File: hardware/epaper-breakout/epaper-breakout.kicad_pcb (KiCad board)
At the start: 2 copper layers, 100 x 40.5 mm, 90 parts, among them J1 XF2M-3315-1A, J2 C10418, J3 Conn_02x06_Counter_Clockwise, J4 ED060SC4, J5 Conn_01x01_Male, J6 Conn_01x01_Male, Q1 AO3401A, Q2 AO3401A, Q3 MMBT3904, Q4 MMBT3904, Q5 AO3401A, Q6 MMBT3904, U1 MCP1700-3302E_SOT23, U10 ED060SC7, U11 TP4056, U12 CH340C, U2 LT1945, U3 LT1945, U4 XC6206PxxxMR, U5 ESP32-WROVER, U6 ED060XC5, U7 LM358, U8 74HC4094-normal, U9 MCP9700AT-ETT

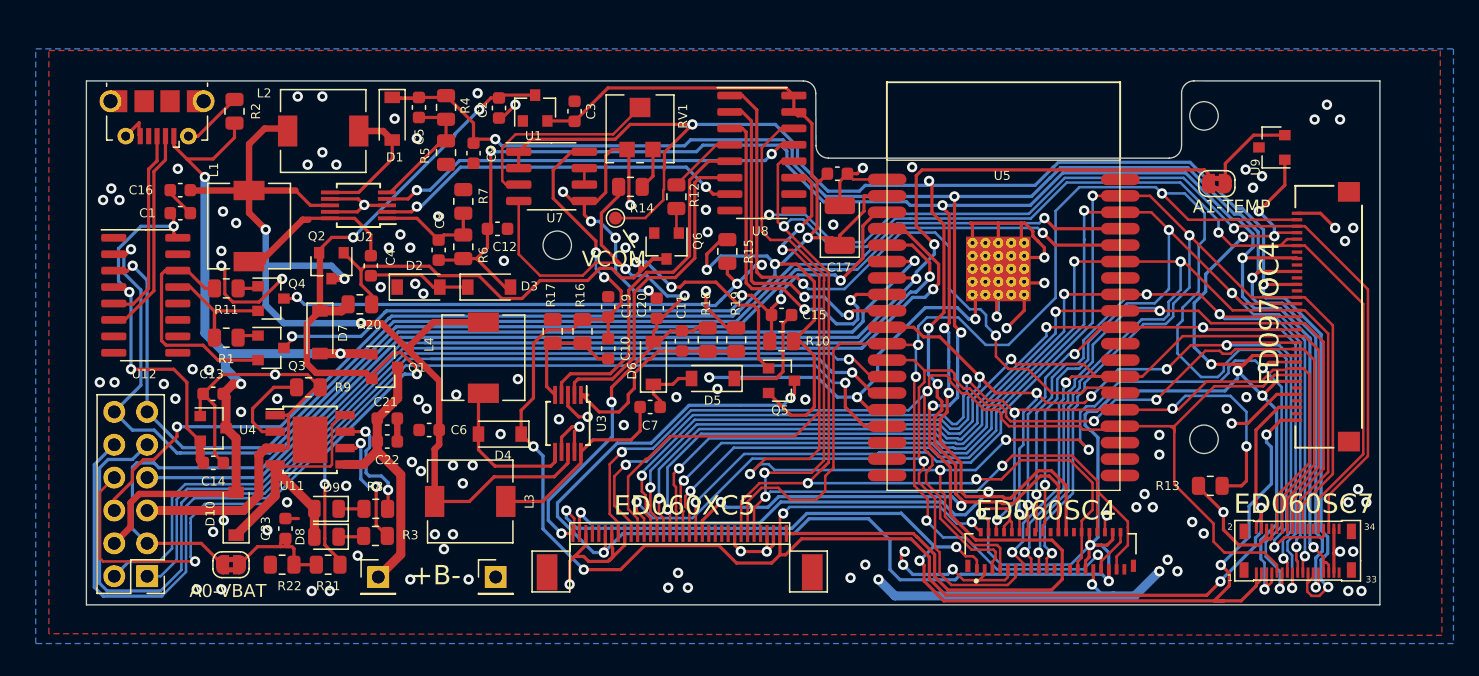
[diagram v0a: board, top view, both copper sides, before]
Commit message: pcb routing
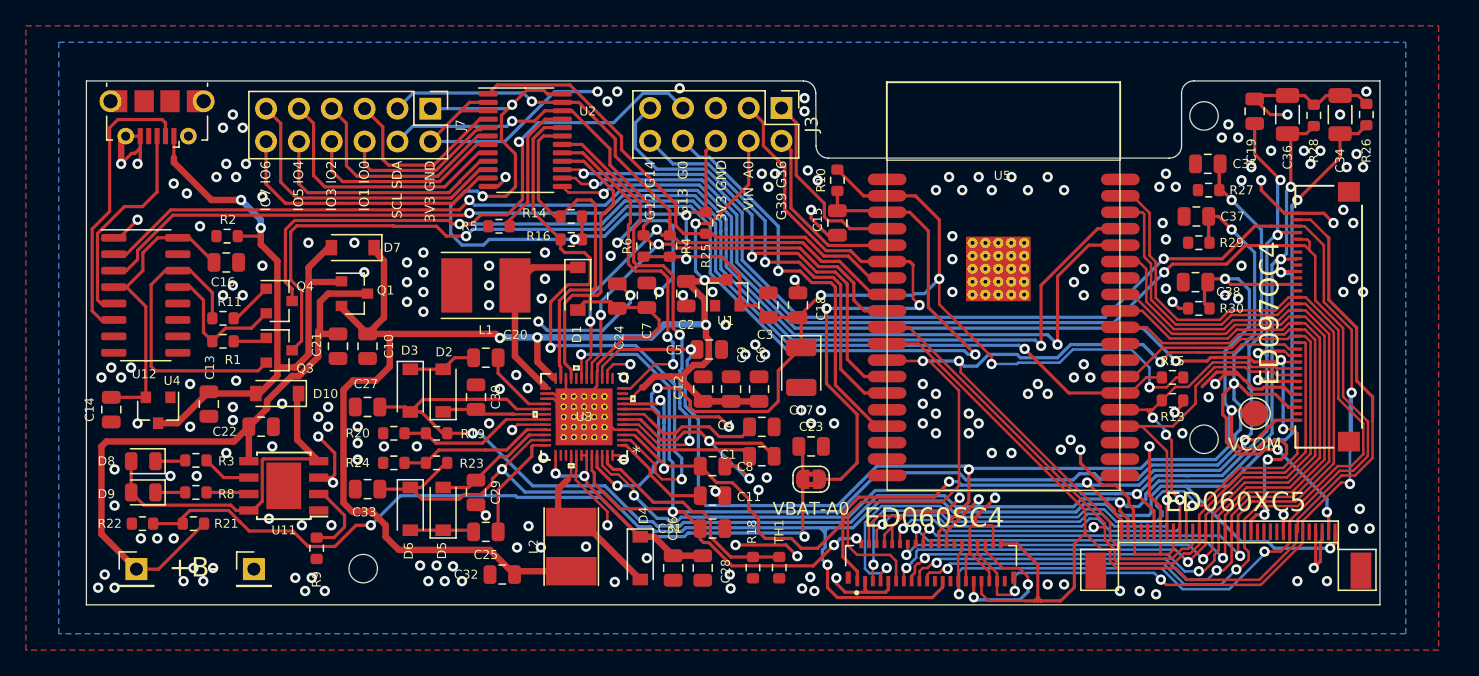
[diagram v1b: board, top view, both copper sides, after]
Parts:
- removed JP_TEMP1: Jumper, Jumper:SolderJumper-2_P1.3mm_Bridged2Bar_RoundedPad1.0x1.5mm
- removed L3, L4: 22uH, Inductor_SMD:L_6.3x6.3_H3
- removed Q2, Q5: AO3401A, Package_TO_SOT_SMD:SOT-23
- removed Q6: MMBT3904, Package_TO_SOT_SMD:SOT-23
- removed R12: 1k, Resistor_SMD:R_0805_2012Metric
- removed R17: 27k, Resistor_SMD:R_0805_2012Metric
- removed R7: 39k, Resistor_SMD:R_0805_2012Metric
- removed RV1: 200k, epaper-breakout:EVM3ESX50B25
- removed TP1: TestPoint_Probe, TestPoint:TestPoint_Pad_D1.0mm
- removed U10: ED060SC7, epaper-breakout:AXT334124
- removed U7: LM358, Package_SO:SOP-8_3.76x4.96mm_P1.27mm
- removed U8: 74HC4094-normal, Package_SO:SOIC-16_3.9x9.9mm_P1.27mm
- removed U9: MCP9700AT-ETT, Package_TO_SOT_SMD:SOT-23
- added C24: 4.7uF, Capacitor_SMD:C_0805_2012Metric, F.Cu at (66.0, 36.1)
- added C25: 10nF, Capacitor_SMD:C_0805_2012Metric, F.Cu at (55.9, 54.4)
- added C26: 4.7uF, Capacitor_SMD:C_0805_2012Metric, F.Cu at (70.4, 57.1)
- added C27: 2.2uF, Capacitor_SMD:C_0805_2012Metric, F.Cu at (46.7, 44.7)
- added C28: 4.7uF, Capacitor_SMD:C_0805_2012Metric, F.Cu at (72.6, 57.1)
- added C29: 100nF, Capacitor_SMD:C_0805_2012Metric, F.Cu at (55.1, 51.3)
- added C30: 100nF, Capacitor_SMD:C_0805_2012Metric, F.Cu at (55.1, 43.9)
- added C31: 4.7uF, Capacitor_SMD:C_0805_2012Metric, F.Cu at (73.4, 54.1)
- added C32: 10uF, Capacitor_SMD:C_0805_2012Metric, F.Cu at (57.1, 57.7)
- added C33: 2.2uF, Capacitor_SMD:C_0805_2012Metric, F.Cu at (46.7, 51.1)
- added C34: 1uF/50V, Capacitor_SMD:C_1206_3216Metric, F.Cu at (121.9, 22.1)
- added C35: 1uF/25V, Capacitor_SMD:C_0805_2012Metric, F.Cu at (111.7, 25.9)
- added C36: 1uF/50V, Capacitor_SMD:C_1206_3216Metric, F.Cu at (117.9, 22.1)
- added C37: 1uF/25V, Capacitor_SMD:C_0805_2012Metric, F.Cu at (110.8, 30.0)
- added C38: 1uF/25V, Capacitor_SMD:C_0805_2012Metric, F.Cu at (110.7, 35.1)
- added J7: Conn_01x12, Connector_PinHeader_2.54mm:PinHeader_2x06_P2.54mm_Vertical, F.Cu at (51.6, 21.6)
- added R23: 1M, Resistor_SMD:R_0603_1608Metric, F.Cu at (52.1, 49.0)
- added R24: 47.5k, Resistor_SMD:R_0603_1608Metric, F.Cu at (48.8, 49.0)
- added R25: 10k, Resistor_SMD:R_0603_1608Metric, F.Cu at (72.9, 30.5)
- added R26: 47k, Resistor_SMD:R_0603_1608Metric, F.Cu at (124.0, 22.1)
- added R27: 47k, Resistor_SMD:R_0603_1608Metric, F.Cu at (111.8, 27.9)
- added R28: 47k, Resistor_SMD:R_0603_1608Metric, F.Cu at (119.9, 22.2)
- added R29: 47k, Resistor_SMD:R_0603_1608Metric, F.Cu at (111.0, 32.0)
- added R30: 100k, Resistor_SMD:R_0603_1608Metric, F.Cu at (111.0, 37.1)
- added TH1: 10k, Resistor_SMD:R_0603_1608Metric, F.Cu at (78.6, 57.1)
- added TP_VCOM1: VCOM, TestPoint:TestPoint_Pad_D2.0mm, F.Cu at (115.3, 45.2)
- C1, C13, C14, C15, C16, C18, C2, C21, C22, C23, C3: footprint Capacitor_SMD:C_0603_1608Metric -> Capacitor_SMD:C_0805_2012Metric
- C10: value 4.7pF -> 22uF; footprint Capacitor_SMD:C_0603_1608Metric -> Capacitor_SMD:C_0805_2012Metric
- C11, C8: value 100pF -> 4.7uF; footprint Capacitor_SMD:C_0603_1608Metric -> Capacitor_SMD:C_0805_2012Metric
- C12, C19, C9: value 1uF -> 10uF; footprint Capacitor_SMD:C_0603_1608Metric -> Capacitor_SMD:C_0805_2012Metric
- C20: value 1uF -> 10nF; footprint Capacitor_SMD:C_0603_1608Metric -> Capacitor_SMD:C_0805_2012Metric
- C4, C7: value 0.1uF -> 4.7uF; footprint Capacitor_SMD:C_0603_1608Metric -> Capacitor_SMD:C_0805_2012Metric
- C5: value 4.7pF -> 4.7uF; footprint Capacitor_SMD:C_0603_1608Metric -> Capacitor_SMD:C_0805_2012Metric
- C6: value 4.7uF -> 22uF; footprint Capacitor_SMD:C_0603_1608Metric -> Capacitor_SMD:C_0805_2012Metric
- J3: value Conn_02x06_Counter_Clockwise -> Conn_02x05_Counter_Clockwise; footprint Connector_PinHeader_2.54mm:PinHeader_2x06_P2.54mm_Vertical -> Connector_PinHeader_2.54mm:PinHeader_2x05_P2.54mm_Vertical
- L1: value 22uH -> 4.7uH; footprint Inductor_SMD:L_6.3x6.3_H3 -> Inductor_SMD:L_Taiyo-Yuden_NR-50xx_HandSoldering
- L2: value 22uH -> 2.2uH; footprint Inductor_SMD:L_6.3x6.3_H3 -> Inductor_SMD:L_Taiyo-Yuden_NR-40xx_HandSoldering
- R1, R10, R11, R13, R15, R2, R21, R22, R3, R8, R9: footprint Resistor_SMD:R_0805_2012Metric -> Resistor_SMD:R_0603_1608Metric
- R14: value 390k -> 10k; footprint Resistor_SMD:R_0805_2012Metric -> Resistor_SMD:R_0603_1608Metric
- R16: value 300k -> 10k; footprint Resistor_SMD:R_0805_2012Metric -> Resistor_SMD:R_0603_1608Metric
- R18: value 110k -> 43k; footprint Resistor_SMD:R_0805_2012Metric -> Resistor_SMD:R_0603_1608Metric
- R19: value 10k -> 1M; footprint Resistor_SMD:R_0805_2012Metric -> Resistor_SMD:R_0603_1608Metric
- R20: value 10k -> 52.3k; footprint Resistor_SMD:R_0805_2012Metric -> Resistor_SMD:R_0603_1608Metric
- R4: value 2M -> 10k; footprint Resistor_SMD:R_0805_2012Metric -> Resistor_SMD:R_0603_1608Metric
- R5: value 120k -> 0; footprint Resistor_SMD:R_0805_2012Metric -> Resistor_SMD:R_0603_1608Metric
- R6: value 560k -> 10k; footprint Resistor_SMD:R_0805_2012Metric -> Resistor_SMD:R_0603_1608Metric
- U2: value LT1945 -> PCA9555PW; footprint Package_SO:MSOP-10_3x3mm_P0.5mm -> Package_SO:TSSOP-24_4.4x7.8mm_P0.65mm
- U3: value LT1945 -> TPS651851RSLR; footprint Package_SO:MSOP-10_3x3mm_P0.5mm -> tps65185:TPS651851RSLR
- moved J3 61.0 mm to (78.7, 21.6), turned to 270 degrees
- moved C19 52.2 mm to (115.3, 21.8), turned to 90 degrees
- moved C1 49.4 mm to (77.2, 48.5), turned to 0 degrees
- moved JP_BAT1 45.3 mm to (81.0, 50.3), turned to 180 degrees
- moved U6 42.4 mm to (113.3, 54.4)
- moved C23 41.1 mm to (81.0, 47.8), turned to 180 degrees
- moved L2 37.4 mm to (62.5, 55.5), turned to 90 degrees
- moved R15 35.8 mm to (109.0, 42.4), turned to 180 degrees
- moved C4 32.7 mm to (77.2, 46.2), turned to 180 degrees
- moved C5 29.2 mm to (73.2, 40.3), turned to 180 degrees
- moved H2 29.2 mm to (46.4, 57.2)
- moved C9 27.0 mm to (74.8, 43.3)
- moved C8 27.0 mm to (73.4, 49.3), turned to 180 degrees
- moved C6 25.7 mm to (77.0, 43.3), turned to 270 degrees
- moved R19 24.3 mm to (52.1, 46.7), turned to 180 degrees
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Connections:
- C1 pad 1: SW_VIN -> /VNEG_IN
- C10 pad 1: Net-(C10-Pad1) -> GND
- C10 pad 2: /15V -> SW_VIN
- C11 pad 1: Net-(C11-Pad1) -> GND
- C11 pad 2: /-15V -> Net-(C11-Pad2)
- C12 pad 1: GND -> SW_VIN
- C12 pad 2: /-20V -> GND
- C19 pad 1: GND -> EPD_VDD
- C19 pad 2: /15V -> GND
- C2 pad 2: VIN -> SW_VIN
- C20 pad 1: GND -> Net-(C20-Pad1)
- C20 pad 2: /-15V -> Net-(C20-Pad2)
- C4 pad 1: Net-(C4-Pad1) -> GND
- C5 pad 1: Net-(C5-Pad1) -> GND
- C5 pad 2: /+22V -> /EP_VCOM
- C6 pad 1: SW_VIN -> GND
- C6 pad 2: GND -> SW_VIN
- C7 pad 1: Net-(C7-Pad1) -> /VNEG_IN
- C7 pad 2: Net-(C7-Pad2) -> GND
- C8 pad 1: Net-(C8-Pad1) -> GND
- C8 pad 2: /-20V -> /-15V
- C9 pad 1: GND -> SW_VIN
- C9 pad 2: /+22V -> GND
- D1 pad 1: /+22V -> Net-(D1-Pad1)
- D1 pad 2: Net-(D1-Pad2) -> /VNEG_IN
- D2 pad 1: GND -> Net-(C30-Pad1)
- D2 pad 2: Net-(C4-Pad1) -> Net-(C20-Pad1)
- D3 pad 1: Net-(C4-Pad1) -> Net-(C20-Pad1)
- D4 pad 1: /15V -> Net-(C26-Pad2)
- D5 pad 1: GND -> Net-(C25-Pad1)
- D5 pad 2: Net-(C7-Pad1) -> Net-(C29-Pad2)
- D6 pad 1: Net-(C7-Pad1) -> /+22V
- D6 pad 2: /-15V -> Net-(C25-Pad1)
- D7 pad 1: VIN -> SW_VIN
- J3 pad 4: VBUS -> SW_VIN
- J3 pad 7: /A1 -> /IO0
- L1 pad 1: Net-(C4-Pad2) -> Net-(D1-Pad1)
- L1 pad 2: SW_VIN -> GND
- L2 pad 1: Net-(D1-Pad2) -> SW_VIN
- L2 pad 2: SW_VIN -> Net-(D4-Pad2)
- Q1 pad 2: VIN -> SW_VIN
- R14 pad 1: /-15V -> /+3.3V
- R14 pad 2: Net-(R14-Pad2) -> /TPS_PWR_GOOD
- R16 pad 1: /15V -> /+3.3V
- R16 pad 2: Net-(C10-Pad1) -> /TPS_nINT
- R18 pad 1: /-15V -> GND
- R18 pad 2: Net-(C11-Pad1) -> Net-(R18-Pad2)
- R19 pad 1: Net-(C11-Pad1) -> /-20V
- R19 pad 2: GND -> Net-(R19-Pad2)
- R20 pad 1: Net-(Q2-Pad1) -> Net-(R19-Pad2)
- R20 pad 2: VIN -> GND
- R21 pad 1: VIN -> BAT+
- R4 pad 1: /+22V -> /+3.3V
- R4 pad 2: Net-(C5-Pad1) -> /SDA
- R5 pad 1: Net-(C5-Pad1) -> Net-(R5-Pad1)
- R6 pad 1: /-20V -> /+3.3V
- R6 pad 2: Net-(C8-Pad1) -> /SCL
- U1 pad 3: VIN -> SW_VIN
- U2 pad 1: Net-(C8-Pad1) -> /~GPIO_INTR
- U2 pad 10: Net-(C4-Pad2) -> Net-(J7-Pad11)
- U2 pad 2: /CTRL-20V -> GND
- U2 pad 4: /CTRL+22V -> Net-(J7-Pad5)
- U2 pad 5: Net-(C5-Pad1) -> Net-(J7-Pad6)
- U2 pad 6: Net-(D1-Pad2) -> Net-(J7-Pad7)
- U2 pad 7: GND -> Net-(J7-Pad8)
- U2 pad 8: SW_VIN -> Net-(J7-Pad9)
- U2 pad 9: GND -> Net-(J7-Pad10)
- U3 pad 1: Net-(C11-Pad1) -> Net-(C11-Pad2)
- U3 pad 10: Net-(C7-Pad2) -> SW_VIN
- U3 pad 2: /CTRL-15V -> /TPS_nINT
- U3 pad 3: GND -> /-15V
- U3 pad 4: /CTRL+15V -> /VNEG_IN
- U3 pad 5: Net-(C10-Pad1) -> /TPS_WAKEUP
- U3 pad 6: Net-(D4-Pad2) -> GND
- U3 pad 7: GND -> Net-(C4-Pad2)
- U3 pad 8: SW_VIN -> GND
- U3 pad 9: GND -> /-15V
- U5 pad 7: /A1 -> /~GPIO_INTR
- U5 pad 8: Net-(U5-Pad8) -> /SDA
- U5 pad 9: Net-(U5-Pad9) -> /SCL
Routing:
- net /A1: track 100.9 -> 0.00 mm, vias 2 -> 0
- net /SENSOR_VN: track 80.0 -> 14.1 mm, vias 1 -> 0
- net /SENSOR_VP: track 79.9 -> 15.0 mm, vias 1 -> 0
- net /-20V: track 188.8 -> 124.2 mm, vias 8 -> 5
- net GND: track 262.0 -> 198.8 mm, vias 132 -> 231
- net VIN: track 63.1 -> 0.00 mm, vias 4 -> 0
- net /EP_VCOM: track 177.6 -> 115.5 mm, vias 8 -> 6
- net /SDA: track 0.00 -> 61.4 mm, vias 0 -> 3
- net /SCL: track 0.00 -> 61.3 mm, vias 0 -> 3
- net EPD_VDD: track 184.5 -> 127.4 mm, vias 12 -> 8
- net /EP_CKV: track 149.6 -> 93.4 mm, vias 6 -> 0
- net /MISO: track 84.9 -> 32.1 mm
- net Net-(C23-Pad2): track 10.0 -> 62.5 mm, vias 0 -> 2
- net Net-(Q2-Pad1): track 51.1 -> 0.00 mm, vias 2 -> 0
- net /SCLK: track 85.8 -> 35.9 mm
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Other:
- board text added: "3V3 GND"
- board text added: "G12 G14"
- board text added: "G13 G0"
- board text added: "G39 G36"
- board text added: "IO1 IO0"
- board text added: "IO3 IO2"
- board text added: "IO5 IO4"
- board text added: "IO7 IO6"
- board text added: "SCL SDA"
- board text added: "VBAT-A0"
- board text added: "VIN A0"
- board text added: "epdiy v6 by Valentin Roland 2021 Thanks to the epdiy contributors!"
- board text removed: "A0-VBAT"
- board text removed: "A1-TEMP"
- board text removed: "ED060SC7"
- board text removed: "RX TX 14 12 35/Tmp 13 GND 3.3V 34 5V 36 39"
- board text removed: "VCOM"
- board text removed: "epdiy v5 by Valentin Roland 2021 Thanks to the epdiy contributors!"
